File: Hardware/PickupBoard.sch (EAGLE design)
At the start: 31 parts, among them U2 TL074_

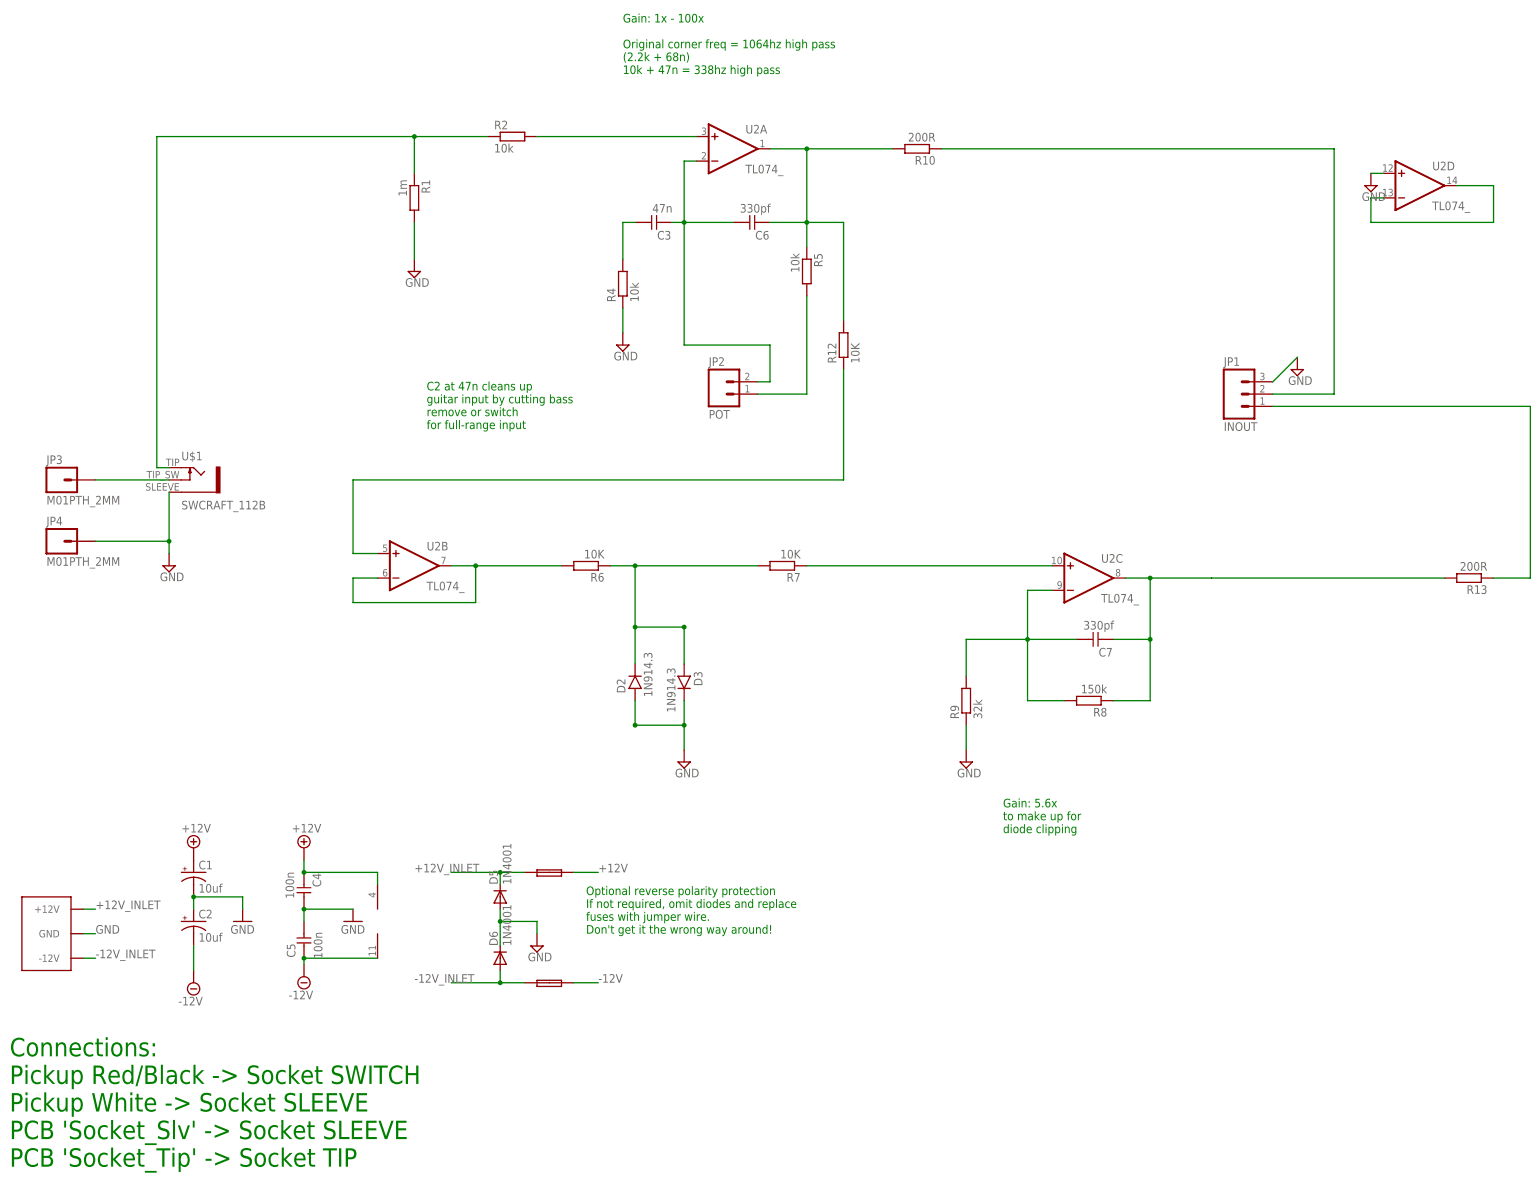
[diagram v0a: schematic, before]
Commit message: Designed and routed
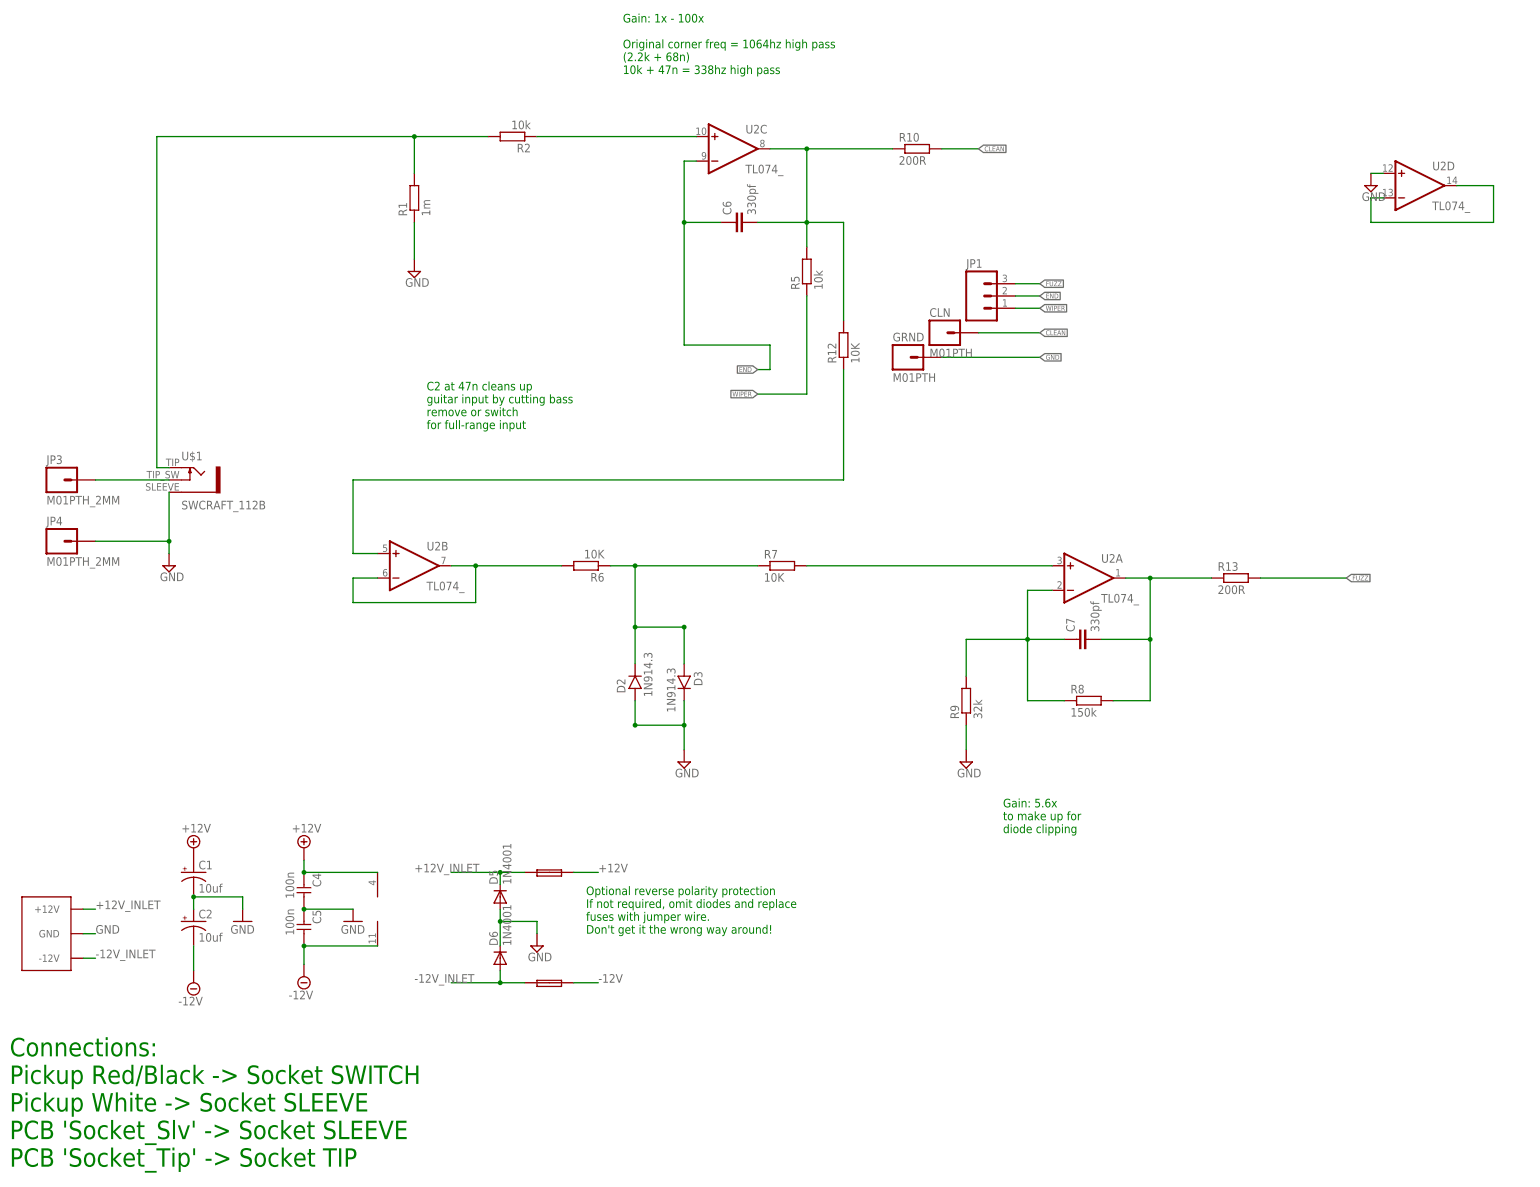
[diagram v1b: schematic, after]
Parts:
- removed C3: 47n, TomW:C-EU050-024X044
- removed JP2: POT, SparkFun-Connectors:M02LOCK
- removed R4: 10k, MusicThingModular:RESISTOR7MM
- added CLN, GRND: M01PTH, SparkFun-Connectors:M01PTH
- C6, C7: device TomW:C-EU050-024X044 -> gm-caps-ceramic:050X030_0251
- JP1: value INOUT -> (none); device SparkFun-Connectors:M03LOCK -> SparkFun-Connectors:M03PTH
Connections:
- removed net N$13: R13.2
- removed net N$16: JP1.2, R10.1
- removed net N$19: JP1.1, R13.1
- removed net N$4: C3.2, C6.1, JP2.2, U2A.-IN
- removed net N$6: JP2.1, R5.2
- removed net N$7: C3.1, R4.2
- new net CLEAN: CLN.1, R10.2
- new net END: C6.1, JP1.2, U2C.-IN
- new net FUZZ: JP1.3, R13.2
- new net WIPER: JP1.1, R5.1
- net -12V: now also C5.1; no longer C5.2
- net GAIN_IN: now also R1.2, R2.2; no longer R1.1, R2.1
- net GND: now also C5.2, GRND.1, R1.1; no longer C5.1, JP1.3, R1.2, R4.1
- net N$11: now also R8.1, U2A.-IN; no longer R8.2, U2C.-IN
- net N$12: now also R13.1, R8.2, U2A.OUT; no longer R8.1, U2C.OUT
- net N$15: now also R10.1, R5.2, U2C.OUT; no longer R10.2, R5.1, U2A.OUT
- net N$2: now also R2.1, U2C.+IN; no longer R2.2, U2A.+IN
- net N$8: now also R7.2, U2A.+IN; no longer R7.1, U2C.+IN
- net N$9: now also R7.1; no longer R7.2
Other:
- moved on the sheet: C5, C6, C7, JP1, R1, R10, R13, R2, R5, R7, R8, U2A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
